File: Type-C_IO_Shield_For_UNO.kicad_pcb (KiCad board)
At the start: 2 copper layers, 68.6 x 53.3 mm, 40 parts, among them J1 USB_C_Receptacle_USB2.0, J10 Conn_01x04, J11 Conn_01x04, J12 Conn_01x04, J13 Conn_01x04, J14 Conn_01x04, J15 Conn_01x04, J16 Conn_Alalog, J17 Conn_01x06, J18 Conn_01x06, J19 Conn_01x06, J2 Conn_01x04, J20 Conn_Digital, J21 Conn_01x04, J22 Conn_01x04, J23 Conn_IIC, J24 Conn_COM, J25 Conn_URF, J26 Conn_SD, J27 Conn_Bluetooth, J3 Conn_01x04, J4 Conn_01x04, J5 Conn_01x04, J6 Conn_01x04, J7 Conn_01x04, J8 Conn_Digital_2, J9 Conn_Power, U1 CH340C

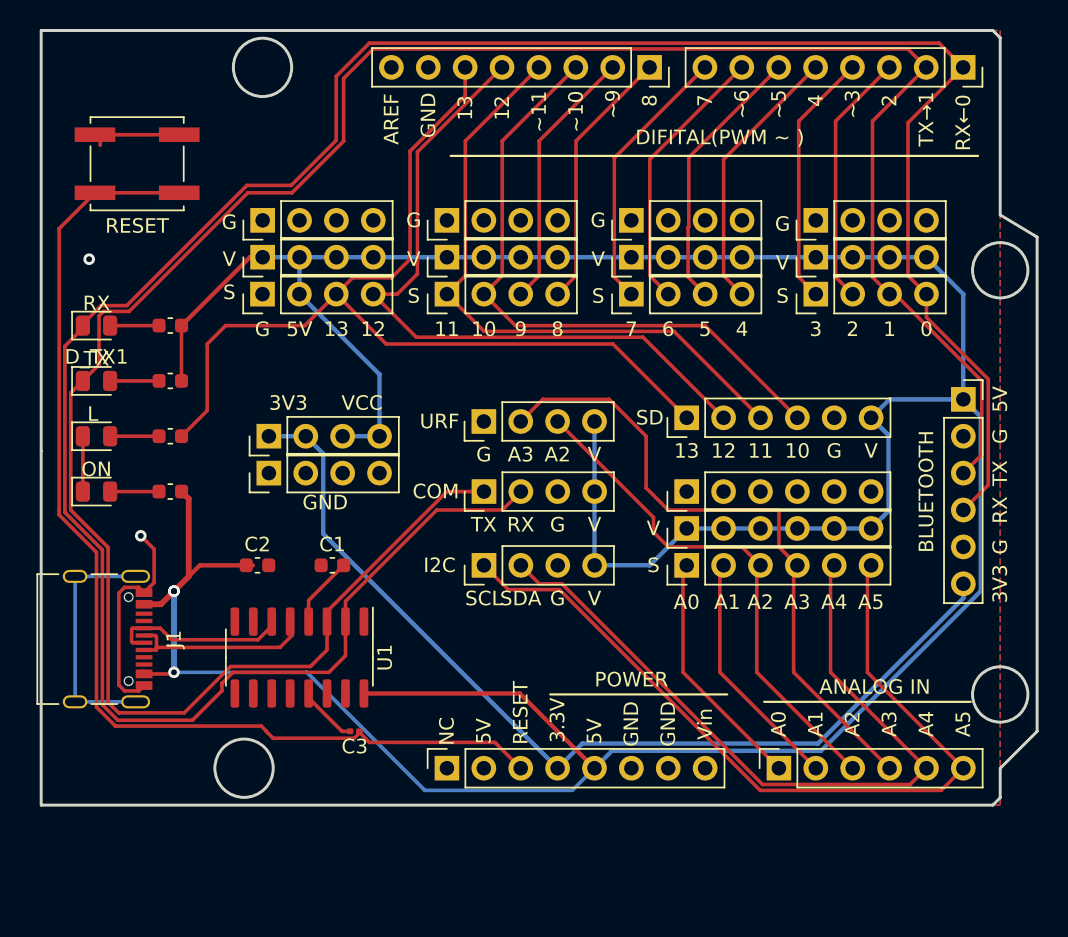
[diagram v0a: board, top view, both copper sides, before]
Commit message: V1.1
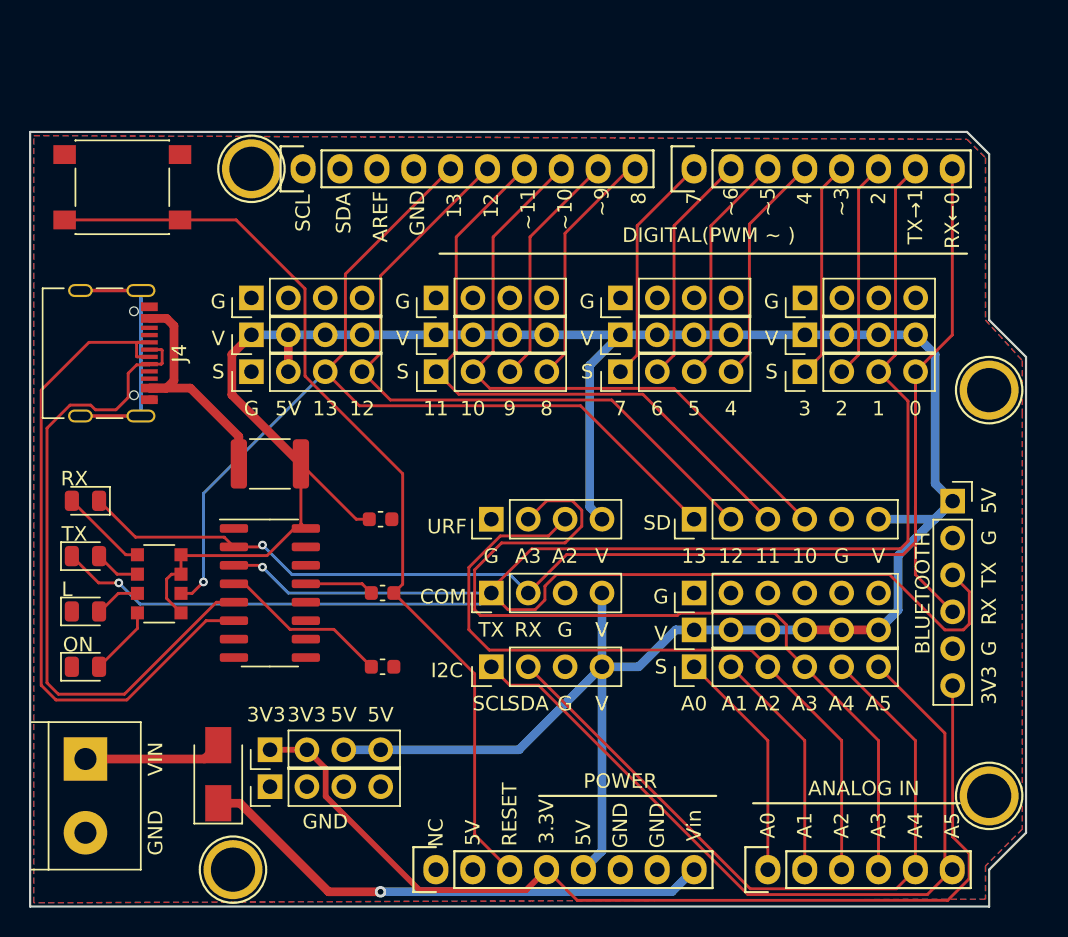
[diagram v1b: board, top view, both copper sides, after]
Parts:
- removed D_L1, D_RX1, D_TX1: LED_YELLOW, LED_SMD:LED_0805_2012Metric
- removed D_ON1: LED_GREEN, LED_SMD:LED_0805_2012Metric
- removed J16: Conn_Alalog, Connector_PinSocket_2.54mm:PinSocket_1x06_P2.54mm_Vertical
- removed J20: Conn_Digital, Connector_PinSocket_2.54mm:PinSocket_1x08_P2.54mm_Vertical
- removed J8: Conn_Digital_2, Connector_PinSocket_2.54mm:PinSocket_1x08_P2.54mm_Vertical
- removed J9: Conn_Power, Connector_PinSocket_2.54mm:PinSocket_1x08_P2.54mm_Vertical
- removed R1, R2, R3, R4: 102, Capacitor_SMD:C_0603_1608Metric
- removed SW_Rest1: RESET, Button_Switch_SMD:SW_Push_1P1T_NO_CK_KSC6xxJ
- added D1: GREEN, LED_SMD:LED_0805_2012Metric, F.Cu at (114.8, 109.9)
- added D2: YELLOW, LED_SMD:LED_0805_2012Metric, F.Cu at (114.8, 106.0)
- added D3: YELLOW, LED_SMD:LED_0805_2012Metric, F.Cu at (114.8, 102.2)
- added D4: YELLOW, LED_SMD:LED_0805_2012Metric, F.Cu at (114.8, 98.4)
- added D5: 1N4007, Diode_SMD:D_SMA, F.Cu at (124.0, 117.3)
- added F1: 0.5A, Fuse:Fuse_1812_4532Metric, F.Cu at (127.5, 95.9)
- added J28: Screw_Terminal_01x02, TerminalBlock:TerminalBlock_bornier-2_P5.08mm, F.Cu at (114.8, 116.2)
- added P1: Power, Socket_Arduino_Uno:Socket_Strip_Arduino_1x08, F.Cu at (138.9, 123.8)
- added P2: Analog, Socket_Arduino_Uno:Socket_Strip_Arduino_1x06, F.Cu at (161.8, 123.8)
- added P3: Digital, Socket_Arduino_Uno:Socket_Strip_Arduino_1x10, F.Cu at (129.8, 75.6)
- added P4: Digital, Socket_Arduino_Uno:Socket_Strip_Arduino_1x08, F.Cu at (156.7, 75.6)
- added P5: CONN_01X01, Socket_Arduino_Uno:Arduino_1pin, F.Cu at (125.0, 123.8)
- added P6: CONN_01X01, Socket_Arduino_Uno:Arduino_1pin, F.Cu at (177.0, 118.7)
- added P7: CONN_01X01, Socket_Arduino_Uno:Arduino_1pin, F.Cu at (126.2, 75.6)
- added P8: CONN_01X01, Socket_Arduino_Uno:Arduino_1pin, F.Cu at (177.0, 90.8)
- added RN1: 102, Resistor_SMD:R_Array_Convex_4x1206, F.Cu at (119.9, 104.1)
- added SW1: SW_SPST, Button_Switch_SMD:SW_Push_1P1T_NO_6x6mm_H9.5mm, F.Cu at (117.3, 76.8)
- C3: footprint Capacitor_SMD:C_0201_0603Metric -> Capacitor_SMD:C_0603_1608Metric
- J1: value USB_C_Receptacle_USB2.0 -> Conn_01x04; footprint Connector_USB:USB_C_Receptacle_Palconn_UTC16-G -> Connector_PinHeader_2.54mm:PinHeader_1x04_P2.54mm_Vertical
- J23: value Conn_IIC -> Conn_01x04
- J24: value Conn_COM -> Conn_01x04
- J25: value Conn_URF -> Conn_01x04
- J26: value Conn_SD -> Conn_01x06
- J27: value Conn_Bluetooth -> Conn_01x06
- J4: value Conn_01x04 -> USB_C_Receptacle_USB2.0; footprint Connector_PinHeader_2.54mm:PinHeader_1x04_P2.54mm_Vertical -> Connector_USB:USB_C_Receptacle_Palconn_UTC16-G
- moved J1 25.5 mm to (126.2, 84.5), turned to 90 degrees
- moved J22 21.6 mm to (127.5, 118.1)
- moved J21 21.6 mm to (127.5, 115.6)
- moved J4 11.1 mm to (116.7, 88.3), turned to -90 degrees
- moved C3 9.72 mm to (135.3, 104.8)
- moved C2 9.05 mm to (135.1, 99.7)
- moved J2 7.92 mm to (126.2, 87.0)
- moved J3 7.92 mm to (126.2, 89.5)
- moved C1 7.79 mm to (135.3, 109.9), turned to 180 degrees
- moved J27 7.05 mm to (174.5, 98.5)
- moved J23 7.00 mm to (142.8, 109.9)
- moved J24 7.00 mm to (142.8, 104.8)
- moved J17 7.00 mm to (156.7, 104.8)
- moved J18 7.00 mm to (156.7, 107.3)
- moved J19 7.00 mm to (156.7, 109.9)
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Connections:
- net 0 renamed /0(Rx)
- net 1 renamed /1(Tx)
- net 10 renamed /10(**/SS)
- net 11 renamed /11(**/MOSI)
- net A2 renamed /A2
- net A3 renamed /A3
- net A4 renamed /A4(SDA)
- net A5 renamed /A5(SCL)
- C2 pad 1: VCC -> +5V
- C3 pad 1: RESET -> /Reset
- J11 pad 1: VCC -> +5V
- J11 pad 2: VCC -> +5V
- J11 pad 3: VCC -> +5V
- J11 pad 4: VCC -> +5V
- J12 pad 1: 7 -> /7
- J12 pad 2: 6 -> /6(**)
- J12 pad 3: 5 -> /5(**)
- J12 pad 4: 4 -> /4
- J14 pad 1: VCC -> +5V
- J14 pad 2: VCC -> +5V
- J14 pad 3: VCC -> +5V
- J14 pad 4: VCC -> +5V
- J15 pad 1: 3 -> /3(**)
- J15 pad 2: 2 -> /2
- J18 pad 1: VCC -> +5V
- J18 pad 2: VCC -> +5V
- J18 pad 3: VCC -> +5V
- J18 pad 4: VCC -> +5V
- J18 pad 5: VCC -> +5V
- J18 pad 6: VCC -> +5V
- J19 pad 1: A0 -> /A0
- J19 pad 2: A1 -> /A1
- J2 pad 1: GND -> +5V
- J2 pad 2: GND -> +5V
- J2 pad 3: GND -> +5V
- J2 pad 4: GND -> +5V
- J21 pad 3: VCC -> +5V
- J21 pad 4: VCC -> +5V
- J23 pad 4: VCC -> +5V
- J24 pad 4: VCC -> +5V
- J25 pad 4: VCC -> +5V
- J26 pad 1: 13 -> /13(SCK)
- J26 pad 2: 12 -> /12(MISO)
- J26 pad 6: VCC -> +5V
- J27 pad 1: VCC -> +5V
- J3 pad 1: VCC -> GND
- J3 pad 2: VCC -> +5V
- J3 pad 3: VCC -> /13(SCK)
- J3 pad 4: VCC -> /12(MISO)
- J6 pad 1: VCC -> +5V
- J6 pad 2: VCC -> +5V
- J6 pad 3: VCC -> +5V
- J6 pad 4: VCC -> +5V
- J7 pad 3: 9 -> /9(**)
- J7 pad 4: 8 -> /8
- U1 pad 16: VCC -> +5V
- U1 pad 5: Net-(J1-PadA6) -> Net-(J4-PadA6)
- U1 pad 6: Net-(J1-PadA7) -> Net-(J4-PadA7)
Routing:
- net VCC: track 251.6 -> 0.00 mm, vias 3 -> 0
- net +5V: track 0.00 -> 187.9 mm
- net RESET: track 74.8 -> 0.00 mm
- net /0(Rx): track 172.9 -> 104.8 mm, vias 0 -> 1
- net /13(SCK): track 0.00 -> 67.0 mm, vias 0 -> 1
- net 13: track 65.9 -> 0.00 mm
- net /Reset: track 0.00 -> 64.9 mm
- net 12: track 47.9 -> 0.00 mm
- net Net-(J4-PadA7): track 0.00 -> 47.8 mm
- net /12(MISO): track 0.00 -> 47.2 mm
- net Net-(J4-PadA6): track 0.00 -> 46.2 mm
- net /Vin: track 0.00 -> 35.9 mm, vias 0 -> 1
- net GND: track 25.5 -> 0.28 mm, vias 2 -> 0
- net 6: track 18.8 -> 0.00 mm
- net 4: track 18.8 -> 0.00 mm
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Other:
- outline, holes or cut-outs redrawn
- board text added: "DIGITAL(PWM ~ )"
- board text added: "VIN"
- board text removed: "DIFITAL(PWM ~ )"
- board text removed: "VCC"
